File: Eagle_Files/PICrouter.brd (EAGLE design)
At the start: 100 x 34 mm, 82 parts, among them IC1 PIC32MX675F512H, IC2 48M033F, IC3 DP83848, IC4 TPS2111A, J1 POWER_JACK, Q1 20MHz, U2 DEVICE, X2 USB-A-H

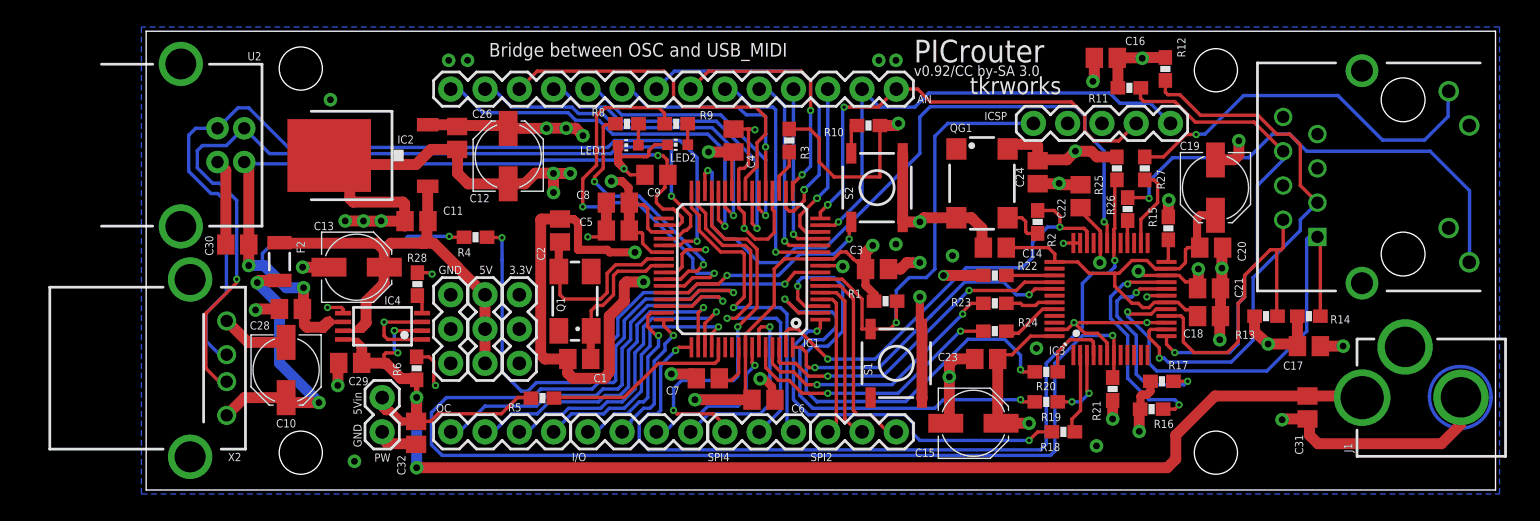
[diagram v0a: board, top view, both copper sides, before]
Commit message: Released PICrouter schematic and board v0.93.
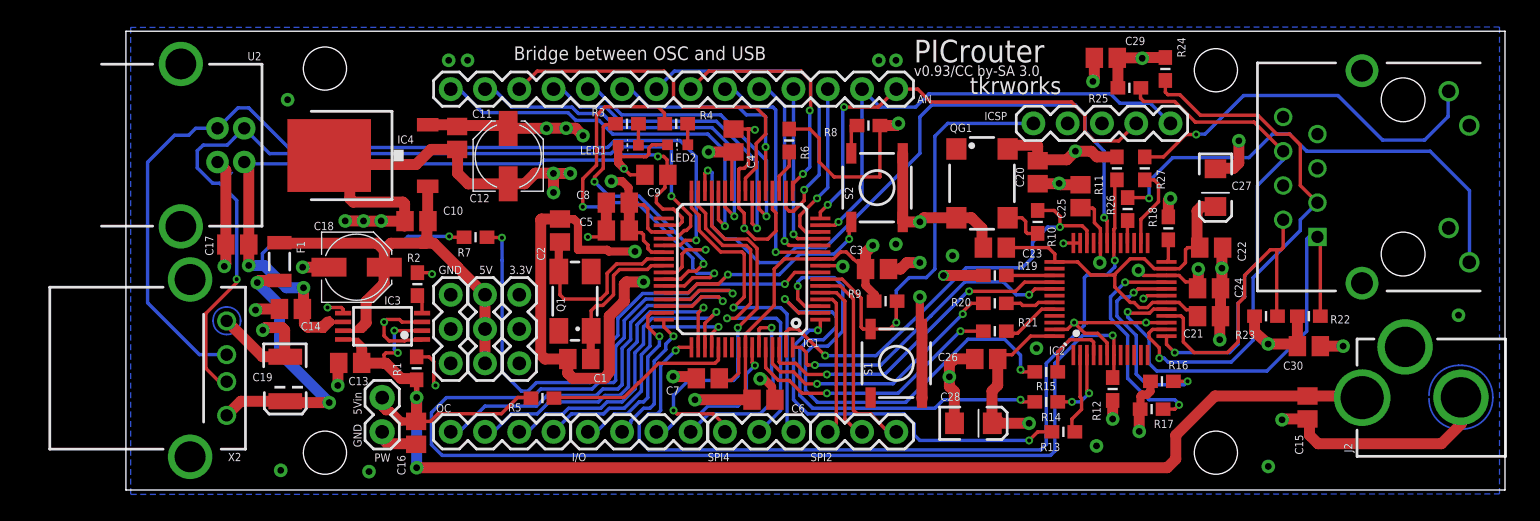
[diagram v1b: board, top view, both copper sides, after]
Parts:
- removed C31, C32: 0.1uF, rcl:C2012
- removed R28: 400, SparkFun:0603-RES
- added C25: 0.1uF, rcl:C2012
- added C27: 10uF, SparkFun:EIA3216
- added R7: 10k, SparkFun:0603-RES
- added U$1: (no value), tkrworks:LOGO
- C10: value 150uF -> 0.1uF; device rcl:PANASONIC_C -> rcl:C2012
- C13: value 100uF -> 0.1uF; device rcl:PANASONIC_C -> rcl:C2012
- C15: value 10uF -> 0.1uF; device rcl:PANASONIC_C -> rcl:C2012
- C17: value 0.1uF -> 10uF
- C18: value 0.1uF -> 100uF; device rcl:C2012 -> rcl:PANASONIC_C
- C19: value 10uF -> 150uF; device rcl:PANASONIC_C -> SparkFun:EIA3528
- C28: value 0.1uF -> 10uF; device rcl:C2012 -> SparkFun:EIA3216
- C30: value 10uF -> 0.1uF
- IC2: value 48M033F -> DP83848; device linear:TO252 -> national-semiconductor:LQFP48
- IC3: value DP83848 -> TPS2111A; device national-semiconductor:LQFP48 -> SparkFun:TSSOP8
- IC4: value TPS2111A -> 48M033F; device SparkFun:TSSOP8 -> linear:TO252
- J1: value POWER_JACK -> (none); device SparkFun:POWER_JACK_PTH_LOCK -> pulse_j0011:PJ-J0
- J2: value (none) -> POWER_JACK; device pulse_j0011:PJ-J0 -> SparkFun:POWER_JACK_PTH_LOCK
- R10: value 10k -> 33
- R11, R12: value 49.9 -> 1.5k
- R13, R14: value 49.9 -> 33
- R15: value 4.87k -> 33
- R18: value 33 -> 4.87k
- R19: value 33 -> 2.2k
- R2: value 33 -> 400
- R21: value 1.5k -> 33
- R22: value 2.2k -> 49.9
- R23, R24: value 33 -> 49.9
- R25: value 1.5k -> 49.9
- R3: value 100 -> 330
- R4: value 10k -> 330
- R6: value 10k -> 100
- R8, R9: value 330 -> 10k
- moved C17 79.8 mm to (8.55, 18.2), turned to 180 degrees
- moved C30 79.8 mm to (88.0, 10.7), turned to 0 degrees
- moved C19 70.4 mm to (12.1, 8.23)
- moved C18 63.3 mm to (17.4, 16.5)
- moved C29 60.4 mm to (72.9, 32.0)
- moved C16 58.2 mm to (21.8, 4.23), turned to 270 degrees
- moved IC2 56.4 mm to (73.3, 14.2)
- moved IC3 54.0 mm to (19.3, 12.1), turned to 180 degrees
- moved C14 52.4 mm to (12.5, 13.4)
- moved C28 51.3 mm to (63.1, 4.94), turned to 0 degrees
- moved R2 46.2 mm to (21.9, 15.3), turned to 270 degrees
- moved C26 42.5 mm to (64.1, 9.71), turned to 180 degrees
- moved R1 35.1 mm to (21.8, 9.02), turned to 270 degrees
- moved R6 32.4 mm to (49.5, 25.9)
- moved C15 24.8 mm to (87.9, 6.12), turned to 270 degrees
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- renumbered F2 to F1
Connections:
- net ECRSDV: now also IC2.40; no longer IC3.40
- net EINT: now also IC2.7, R12.1; no longer IC3.7, R21.1
- net EMDC: now also IC2.31; no longer IC3.31
- net EMDIO: now also IC2.30, R11.2; no longer IC3.30, R25.2
- net EREFCLK: now also IC2.34, R10.2; no longer IC3.34, R2.2
- net ERXD0: now also R20.1; no longer R23.1
- net ERXD1: now also R21.1; no longer R24.1
- net ERXERR: now also IC2.41; no longer IC3.41
- net ETXD0: now also R14.1; no longer R19.1
- net ETXD1: now also R15.1; no longer R20.1
- net ETXEN: now also R13.1; no longer R18.1
- net GND: now also C10.2, C13.2, C15.2, C18.-, C19.C, C25.2, C27.C, C28.C, IC2.15, IC2.19, IC2.35, IC2.36, IC2.47, IC2.6, IC3.1, IC3.3, IC3.5, J1.10, J1.11, J1.8, J1.S1, J1.S2, J2.GND, R1.1, R18.2, R2.1; no longer C10.-, C13.-, C15.-, C18.2, C19.-, C28.2, C31.2, C32.2, IC2.3, IC3.15, IC3.19, IC3.35, IC3.36, IC3.47, IC3.6, IC4.1, IC4.5, J1.GND, J2.10, J2.11, J2.8, J2.S1, J2.S2, R15.2, R28.1, R6.1
- net LED_ACT: now also IC2.26; no longer IC3.26
- net LED_LINK: now also IC2.28; no longer IC3.28
- net N$10: now also R6.2; no longer R3.2
- net N$12: now also R7.2; no longer R4.2
- net N$13: now also R3.2; no longer R8.2
- net N$14: now also R4.2; no longer R9.2
- net N$15: now also R3.1; no longer R8.1
- net N$16: now also R4.1; no longer R9.1
- net N$47: now also IC2.21, R17.1; no longer IC3.21, R16.1
- net N$48: now also IC2.20, R16.1; no longer IC3.20, R17.1
- net N$49: now also IC2.39, R19.2; no longer IC3.39, R22.2
- net N$52: now also IC2.4, R15.2; no longer IC3.4, R20.2
- net N$53: now also IC2.3, R14.2; no longer IC3.3, R19.2
- net N$54: now also IC2.2, R13.2; no longer IC3.2, R18.2
- net N$55: now also J1.9; no longer J2.9
- net N$56: now also IC2.43, R20.2; no longer IC3.43, R23.2
- net N$57: now also IC2.44, R21.2; no longer IC3.44, R24.2
- net N$58: now also R10.1; no longer R2.1
- net N$6: now also R9.1; no longer R1.1
- net N$61: now also IC3.4, R2.2; no longer IC4.4, R28.2
- net N$62: now also J1.12; no longer J2.12
- net N$8: now also R8.1; no longer R10.1
- net N$9: now also IC2.24, R18.1; no longer IC3.24, R15.1
- net PFBOUT: now also C21.1, C22.1, C23.1, C27.A, IC2.18, IC2.23, IC2.37; no longer C14.1, C18.1, C19.+, C20.1, IC3.18, IC3.23, IC3.37
- net RDM: now also IC2.13, J1.6, R25.1; no longer IC3.13, J2.6, R11.1
- net RDP: now also IC2.14, J1.3, R24.1; no longer IC3.14, J2.3, R12.1
- net SELF: now also C13.1, C15.1, C16.1, IC3.2, IC3.8, J2.PWR, R1.2; no longer C29.1, C31.1, C32.1, IC4.2, IC4.8, J1.PWR, R6.2
- net TDM: now also IC2.16, J1.2, R23.1; no longer IC3.16, J2.2, R13.1
- net TDP: now also IC2.17, J1.1, R22.1; no longer IC3.17, J2.1, R14.1
- net VBUS: now also C14.1, C17.1, IC3.6, R7.1; no longer C28.1, C30.1, IC4.6, R4.1
- net VBUS_HOST: now also C19.A; no longer C10.+
- net VCC: now also C10.1, C18.+, IC3.7, IC4.1; no longer C11.1, C13.+, IC2.1, IC4.7
- net VDD: now also C11.1, C20.1, C25.1, C28.A, C29.1, C30.1, IC2.22, IC2.32, IC2.48, IC4.2, J1.4, J1.5, R11.1, R19.1, R22.2, R23.2, R24.2, R25.2, R6.1, R8.2, R9.2; no longer C15.+, C16.1, C17.1, C21.1, C22.1, C23.1, IC2.2, IC3.22, IC3.32, IC3.48, J2.4, J2.5, R1.2, R10.2, R11.2, R13.2, R14.2, R21.2, R22.1, R25.1, R3.1
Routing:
- net GND: track 220.9 -> 228.1 mm, vias 49 -> 54
- net N$67: track 0.00 -> 7.03 mm
- net N$70: track 0.00 -> 5.79 mm
- net N$69: track 0.00 -> 5.76 mm
- net D+: track 68.6 -> 70.9 mm
- net VDD: track 127.2 -> 129.2 mm
- net VBUS_HOST: track 20.0 -> 20.9 mm
- net N$68: track 0.00 -> 0.80 mm
- net PFBOUT: track 29.4 -> 30.2 mm
- net N$5: track 12.8 -> 13.3 mm
- net N$4: vias 3 -> 2
- net SELF: vias 5 -> 4
- net N$23: vias 2 -> 1
- net N$18: vias 2 -> 1
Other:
- board size 100 x 34 mm -> 102.2 x 34 mm
- board text added: "Bridge between OSC and USB"
- board text added: "v0.93/CC by-SA 3.0"
- board text removed: "Bridge between OSC and USB_MIDI"
- board text removed: "v0.92/CC by-SA 3.0"

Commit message: Released PICrouter schematic and board v0.94.
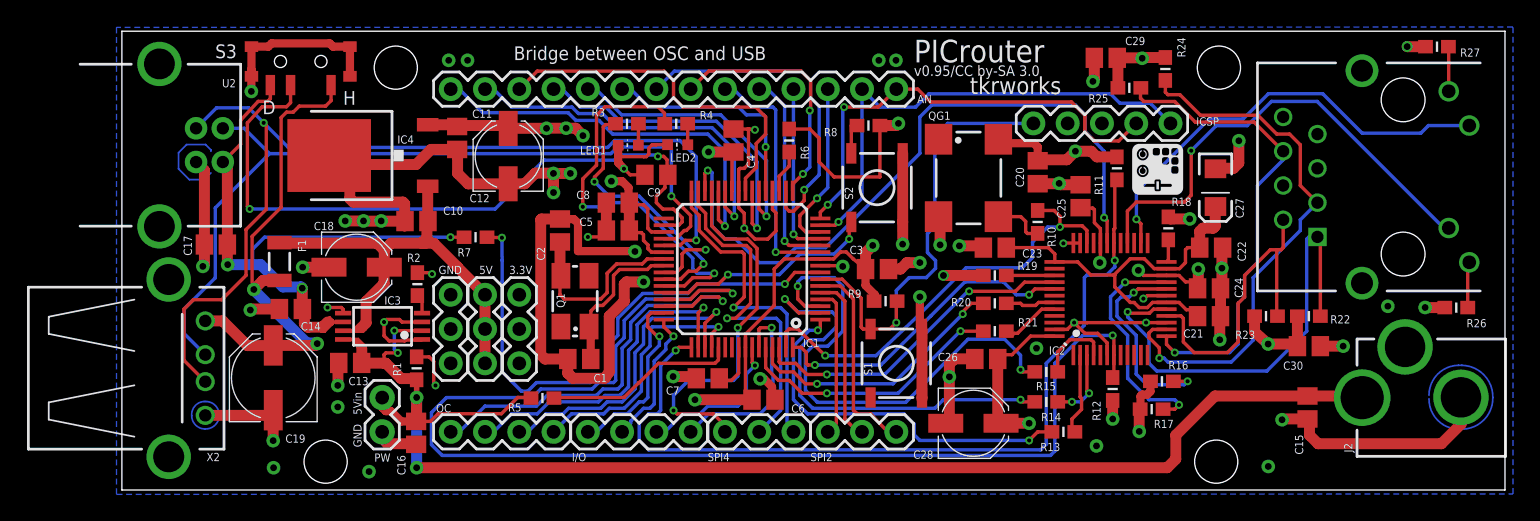
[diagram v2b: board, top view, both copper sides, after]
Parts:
- added S3: SSSS810701-1-2, alps_japan_potentiometers:SSSS810701
- C19: value 150uF -> 220uF; device SparkFun:EIA3528 -> rcl:PANASONIC_D
- C28: device SparkFun:EIA3216 -> rcl:PANASONIC_C
- Q1: device crystal:CTS406 -> my-crystal:CTS406
- QG1: value SM77H -> 50MHz; device crystal:SM77H -> my-crystal:SM77H
- moved U$1 56.9 mm to (74.9, 21.9)
- moved R26 25.4 mm to (98.9, 13.5), turned to 0 degrees
- moved R27 23.5 mm to (97.5, 32.9), turned to 0 degrees
- moved C17 1.59 mm to (6.97, 18.2)
- moved X2 1.59 mm to (3.47, 9.03)
- moved U2 1.59 mm to (5.50, 25.6)
- moved QG1 1.08 mm to (62.7, 23.1)
- moved C19 0.89 mm to (11.2, 8.31), turned to 90 degrees
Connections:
- new net VBUS_DEVICE: C14.1, C17.1, IC3.6, R7.1, S3.P$3, U2.VBUS
- net GND: now also C19.-, C28.-, S3.P$4, S3.P$5, S3.P$6, S3.P$7; no longer C19.C, C28.C, J1.10, J1.11
- net LED_ACT: now also J1.11; no longer R27.1
- net LED_LINK: now also J1.10; no longer R26.1
- net VBUS: now also S3.P$2; no longer C14.1, C17.1, IC3.6, R7.1, U2.VBUS
- net VBUS_HOST: now also C19.+, S3.P$1; no longer C19.A
- net VDD: now also C28.+, R26.1, R27.1; no longer C28.A
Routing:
- net VBUS_DEVICE: track 0.00 -> 44.7 mm, vias 0 -> 3
- net LED_LINK: track 1.68 -> 35.4 mm, vias 0 -> 1
- net N$55: track 35.1 -> 3.41 mm, vias 1 -> 0
- net LED_ACT: track 6.05 -> 33.1 mm, vias 0 -> 1
- net N$62: track 28.3 -> 3.31 mm, vias 1 -> 0
- net VBUS: track 74.4 -> 52.0 mm, vias 4 -> 2
- net VBUS_HOST: track 20.9 -> 36.7 mm
- net GND: track 228.1 -> 239.7 mm, vias 54 -> 55
- net N$71: track 0.00 -> 7.05 mm
- net D-: track 66.1 -> 61.2 mm, vias 2 -> 1
- net VDD: track 129.2 -> 132.0 mm, vias 18 -> 20
- net D+: track 70.9 -> 72.0 mm, vias 1 -> 2
- net N$68: track 0.80 -> 0.00 mm
- net N$58: track 3.16 -> 3.88 mm
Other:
- board size 102.2 x 34 mm -> 102.5 x 34 mm
- board text added: "D"
- board text added: "H"
- board text added: "v0.95/CC by-SA 3.0"
- board text removed: "v0.93/CC by-SA 3.0"
